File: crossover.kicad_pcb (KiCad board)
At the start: 2 copper layers, 99.7 x 90.8 mm, 86 parts, among them J1 Power In, J2 Line In, J3 Tweeter Out, J4 Sub Out, U1 TL072, U2 TL072, U3 TL072, U4 TL072, U5 TL072, U6 TL072, U7 TL072

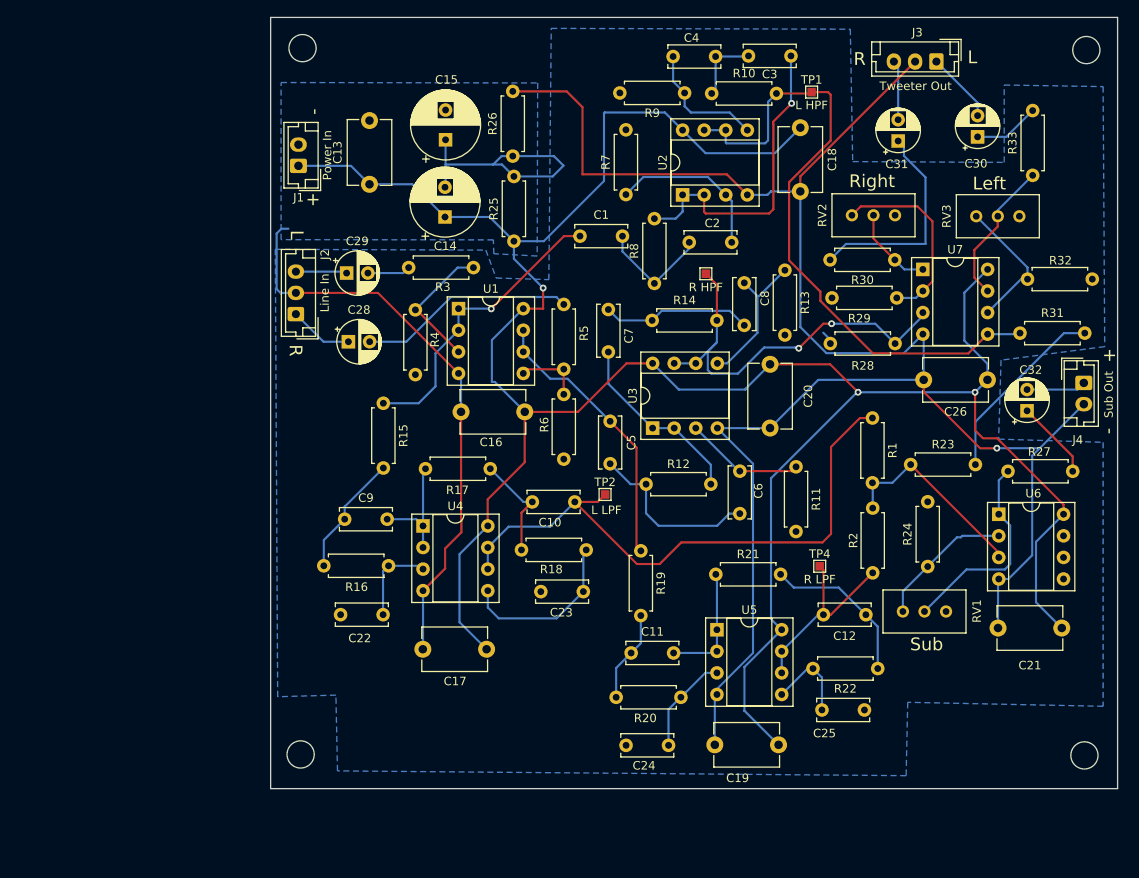
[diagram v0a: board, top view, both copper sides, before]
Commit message: Finish placing
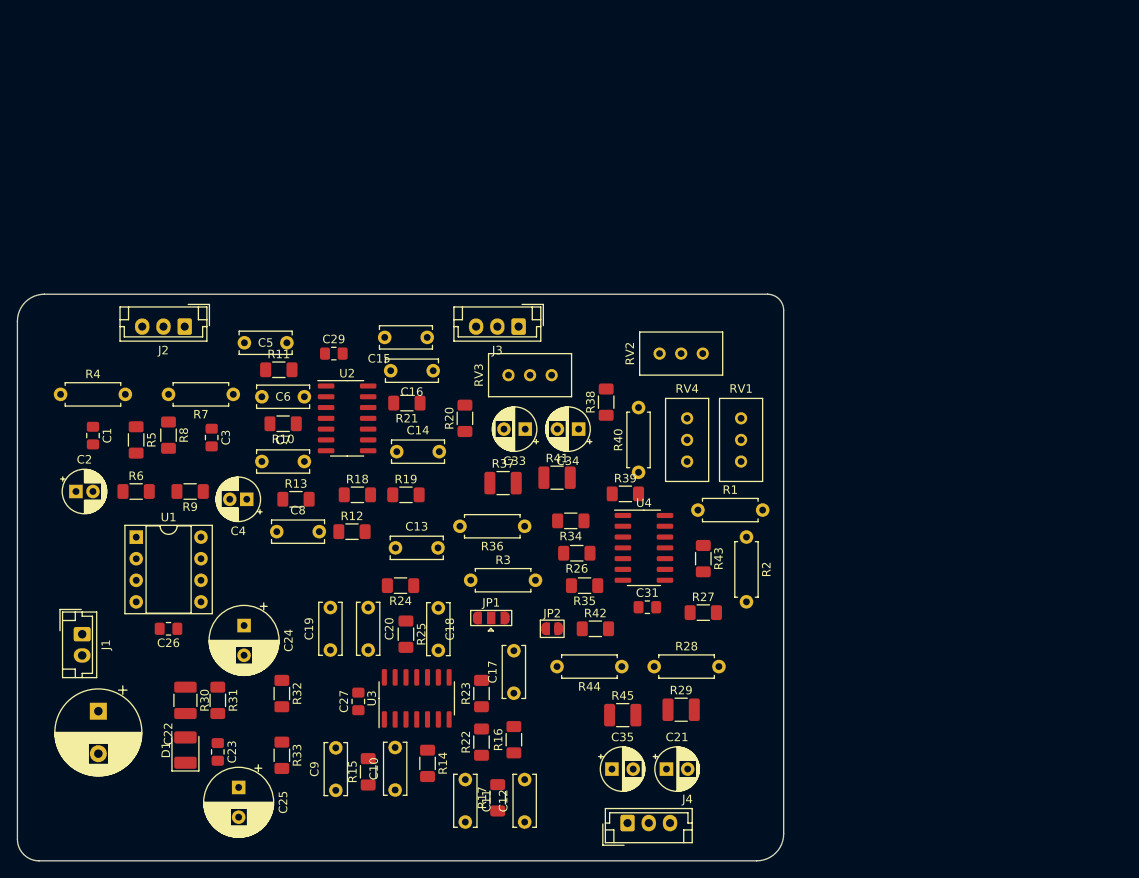
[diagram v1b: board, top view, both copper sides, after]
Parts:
- removed C28, C30, C32: 2.2u, Capacitor_THT:CP_Radial_D5.0mm_P2.50mm
- removed REF** (x4): MountingHole_3.2mm_M3, MountingHole:MountingHole_3.2mm_M3
- removed TP1: L HPF, TestPoint:TestPoint_Pad_1.0x1.0mm
- removed TP2: L LPF, TestPoint:TestPoint_Pad_1.0x1.0mm
- removed TP3: R HPF, TestPoint:TestPoint_Pad_1.0x1.0mm
- removed TP4: R LPF, TestPoint:TestPoint_Pad_1.0x1.0mm
- removed U5, U6, U7: TL072, Package_DIP:DIP-8_W7.62mm_Socket
- added C27: 100n, Capacitor_SMD:C_0805_2012Metric_Pad1.18x1.45mm_HandSolder, F.Cu at (73.1, 107.0)
- added C33: 2.2U, Capacitor_THT:CP_Radial_D5.0mm_P2.50mm, F.Cu at (92.8, 74.9)
- added C34: 2.2U, Capacitor_THT:CP_Radial_D5.0mm_P2.50mm, F.Cu at (99.1, 74.9)
- added C35: 2.2U, Capacitor_THT:CP_Radial_D5.0mm_P2.50mm, F.Cu at (103.0, 114.9)
- added D1: LED, LED_SMD:LED_1210_3225Metric_Pad1.42x2.65mm_HandSolder, F.Cu at (52.8, 112.7)
- added JP1: Sub Stereo/Mono, Jumper:SolderJumper-3_P1.3mm_Open_RoundedPad1.0x1.5mm, F.Cu at (88.8, 97.2)
- added JP2: Sub Mono, Jumper:SolderJumper-2_P1.3mm_Open_RoundedPad1.0x1.5mm, F.Cu at (96.0, 98.4)
- added R34: 10k, Resistor_SMD:R_1206_3216Metric_Pad1.30x1.75mm_HandSolder, F.Cu at (98.1, 85.7)
- added R35: 10K, Resistor_SMD:R_1206_3216Metric_Pad1.30x1.75mm_HandSolder, F.Cu at (99.8, 93.3)
- added R36: 100, Resistor_THT:R_Axial_DIN0207_L6.3mm_D2.5mm_P7.62mm_Horizontal, F.Cu at (92.7, 86.4)
- added R37: 4.7K, Resistor_SMD:R_1210_3225Metric_Pad1.30x2.65mm_HandSolder, F.Cu at (90.2, 81.3)
- added R38: 10k, Resistor_SMD:R_1206_3216Metric_Pad1.30x1.75mm_HandSolder, F.Cu at (102.3, 71.8)
- added R39: 10K, Resistor_SMD:R_1206_3216Metric_Pad1.30x1.75mm_HandSolder, F.Cu at (104.6, 82.5)
- added R40: 100, Resistor_THT:R_Axial_DIN0207_L6.3mm_D2.5mm_P7.62mm_Horizontal, F.Cu at (106.1, 80.0)
- added R41: 4.7K, Resistor_SMD:R_1210_3225Metric_Pad1.30x2.65mm_HandSolder, F.Cu at (96.5, 80.6)
- added R42: 10k, Resistor_SMD:R_1206_3216Metric_Pad1.30x1.75mm_HandSolder, F.Cu at (101.0, 98.4)
- added R43: 10K, Resistor_SMD:R_1206_3216Metric_Pad1.30x1.75mm_HandSolder, F.Cu at (113.7, 90.2)
- added R44: 100, Resistor_THT:R_Axial_DIN0207_L6.3mm_D2.5mm_P7.62mm_Horizontal, F.Cu at (104.1, 102.9)
- added R45: 4.7K, Resistor_SMD:R_1210_3225Metric_Pad1.30x2.65mm_HandSolder, F.Cu at (104.2, 108.6)
- added RV4: 10K, Potentiometer_THT:Potentiometer_Bourns_3386C_Horizontal, F.Cu at (111.8, 73.7)
- C1, C3: value 33nf -> 1n; footprint Capacitor_THT:C_Disc_D6.0mm_W2.5mm_P5.00mm -> Capacitor_SMD:C_0805_2012Metric_Pad1.18x1.45mm_HandSolder
- C10, C11, C12, C9: value 66nf -> 33nf
- C13, C17, C19: value 100n -> 33nf; footprint Capacitor_THT:C_Disc_D7.5mm_W5.0mm_P7.50mm -> Capacitor_THT:C_Disc_D6.0mm_W2.5mm_P5.00mm
- C14: value 10u -> 66nf; footprint Capacitor_THT:CP_Radial_D8.0mm_P3.50mm -> Capacitor_THT:C_Disc_D6.0mm_W2.5mm_P5.00mm
- C15: value 10u -> 33nf; footprint Capacitor_THT:CP_Radial_D8.0mm_P3.50mm -> Capacitor_THT:C_Disc_D6.0mm_W2.5mm_P5.00mm
- C16, C18, C20: value 100n -> 66nf; footprint Capacitor_THT:C_Disc_D7.5mm_W5.0mm_P7.50mm -> Capacitor_THT:C_Disc_D6.0mm_W2.5mm_P5.00mm
- C2, C4: value 33nf -> 4.7uF; footprint Capacitor_THT:C_Disc_D6.0mm_W2.5mm_P5.00mm -> Capacitor_THT:CP_Radial_D5.0mm_P2.00mm
- C21: value 100n -> 2.2U; footprint Capacitor_THT:C_Disc_D7.5mm_W5.0mm_P7.50mm -> Capacitor_THT:CP_Radial_D5.0mm_P2.50mm
- C22: value 33nf -> 1000uF; footprint Capacitor_THT:C_Disc_D6.0mm_W2.5mm_P5.00mm -> Capacitor_THT:CP_Radial_D10.0mm_P5.00mm
- C23: value 33nf -> 100n; footprint Capacitor_THT:C_Disc_D6.0mm_W2.5mm_P5.00mm -> Capacitor_SMD:C_0805_2012Metric_Pad1.18x1.45mm_HandSolder
- C24, C25: value 33nf -> 10u; footprint Capacitor_THT:C_Disc_D6.0mm_W2.5mm_P5.00mm -> Capacitor_THT:CP_Radial_D8.0mm_P3.50mm
- C26: footprint Capacitor_THT:C_Disc_D7.5mm_W5.0mm_P7.50mm -> Capacitor_SMD:C_0805_2012Metric_Pad1.18x1.45mm_HandSolder
- C29, C31: value 2.2u -> 100n; footprint Capacitor_THT:CP_Radial_D5.0mm_P2.50mm -> Capacitor_SMD:C_0805_2012Metric_Pad1.18x1.45mm_HandSolder
- J4: footprint Connector_JST:JST_EH_B2B-EH-A_1x02_P2.50mm_Vertical -> Connector_JST:JST_EH_B3B-EH-A_1x03_P2.50mm_Vertical
- R10, R12, R14, R16: value 27K -> 39K; footprint Resistor_THT:R_Axial_DIN0207_L6.3mm_D2.5mm_P7.62mm_Horizontal -> Resistor_SMD:R_1206_3216Metric_Pad1.30x1.75mm_HandSolder
- R11, R13: value 56K -> 20K; footprint Resistor_THT:R_Axial_DIN0207_L6.3mm_D2.5mm_P7.62mm_Horizontal -> Resistor_SMD:R_1206_3216Metric_Pad1.30x1.75mm_HandSolder
- R15, R17, R18, R19, R20, R21, R22: value 27K -> 20K; footprint Resistor_THT:R_Axial_DIN0207_L6.3mm_D2.5mm_P7.62mm_Horizontal -> Resistor_SMD:R_1206_3216Metric_Pad1.30x1.75mm_HandSolder
- R23: value 10k -> 20K; footprint Resistor_THT:R_Axial_DIN0207_L6.3mm_D2.5mm_P7.62mm_Horizontal -> Resistor_SMD:R_1206_3216Metric_Pad1.30x1.75mm_HandSolder
- R24: value 5k -> 20K; footprint Resistor_THT:R_Axial_DIN0207_L6.3mm_D2.5mm_P7.62mm_Horizontal -> Resistor_SMD:R_1206_3216Metric_Pad1.30x1.75mm_HandSolder
- R25: value 10K -> 20K; footprint Resistor_THT:R_Axial_DIN0207_L6.3mm_D2.5mm_P7.62mm_Horizontal -> Resistor_SMD:R_1206_3216Metric_Pad1.30x1.75mm_HandSolder
- R26: value 10K -> 10k; footprint Resistor_THT:R_Axial_DIN0207_L6.3mm_D2.5mm_P7.62mm_Horizontal -> Resistor_SMD:R_1206_3216Metric_Pad1.30x1.75mm_HandSolder
- R27, R33: value 100 -> 10K; footprint Resistor_THT:R_Axial_DIN0207_L6.3mm_D2.5mm_P7.62mm_Horizontal -> Resistor_SMD:R_1206_3216Metric_Pad1.30x1.75mm_HandSolder
- R28: value 10k -> 100
- R29: value 5k -> 4.7K; footprint Resistor_THT:R_Axial_DIN0207_L6.3mm_D2.5mm_P7.62mm_Horizontal -> Resistor_SMD:R_1210_3225Metric_Pad1.30x2.65mm_HandSolder
- R3: value 1K -> 100
- R30: value 100 -> 2.2K; footprint Resistor_THT:R_Axial_DIN0207_L6.3mm_D2.5mm_P7.62mm_Horizontal -> Resistor_SMD:R_1210_3225Metric_Pad1.30x2.65mm_HandSolder
- R31: value 10k -> 1K; footprint Resistor_THT:R_Axial_DIN0207_L6.3mm_D2.5mm_P7.62mm_Horizontal -> Resistor_SMD:R_1206_3216Metric_Pad1.30x1.75mm_HandSolder
- R32: value 5k -> 10K; footprint Resistor_THT:R_Axial_DIN0207_L6.3mm_D2.5mm_P7.62mm_Horizontal -> Resistor_SMD:R_1206_3216Metric_Pad1.30x1.75mm_HandSolder
- R4: value 100K -> 100
- R5: value 1K -> 22K; footprint Resistor_THT:R_Axial_DIN0207_L6.3mm_D2.5mm_P7.62mm_Horizontal -> Resistor_SMD:R_1206_3216Metric_Pad1.30x1.75mm_HandSolder
- R6: value 100K -> 22K; footprint Resistor_THT:R_Axial_DIN0207_L6.3mm_D2.5mm_P7.62mm_Horizontal -> Resistor_SMD:R_1206_3216Metric_Pad1.30x1.75mm_HandSolder
- R7: value 56K -> 100
- R8: value 27K -> 22K; footprint Resistor_THT:R_Axial_DIN0207_L6.3mm_D2.5mm_P7.62mm_Horizontal -> Resistor_SMD:R_1206_3216Metric_Pad1.30x1.75mm_HandSolder
- R9: value 56K -> 22K; footprint Resistor_THT:R_Axial_DIN0207_L6.3mm_D2.5mm_P7.62mm_Horizontal -> Resistor_SMD:R_1206_3216Metric_Pad1.30x1.75mm_HandSolder
- U2, U3, U4: value TL072 -> TL074; footprint Package_DIP:DIP-8_W7.62mm_Socket -> Package_SO:SOIC-14_3.9x8.7mm_P1.27mm
- moved R33 111.6 mm to (64.1, 113.3), turned to -90 degrees
- moved R31 103.8 mm to (56.6, 106.8), turned to -90 degrees
- moved C26 100.7 mm to (50.8, 98.4)
- moved R32 100.4 mm to (64.1, 106.0), turned to -90 degrees
- moved R30 98.3 mm to (52.8, 106.8), turned to -90 degrees
- moved C3 81.6 mm to (55.9, 75.9), turned to -90 degrees
- moved C2 77.9 mm to (39.9, 82.3)
- moved C4 75.9 mm to (60.0, 83.2)
- moved C18 74.8 mm to (82.5, 101.0), turned to 90 degrees
- moved R9 74.7 mm to (53.3, 82.3)
- moved J4 74.6 mm to (104.8, 121.3), turned to 0 degrees
- moved C25 74.2 mm to (59.1, 117.1), turned to -90 degrees
- moved R10 63.7 mm to (64.3, 74.3), turned to 180 degrees
- moved R13 63.5 mm to (65.8, 83.2), turned to 0 degrees
- moved C31 62.3 mm to (107.1, 95.9), turned to 0 degrees
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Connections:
- C1 pad 1: /Left HPF/in -> Net-(C1-Pad1)
- C1 pad 2: Net-(C1-Pad2) -> VDD
- C10 pad 2: /Left LPF/out -> Net-(U3A-+)
- C11 pad 1: Net-(C11-Pad1) -> /Right HPF/HPF Stage 2/in
- C11 pad 2: /Right LPF/LPF Stage 1/out -> Net-(C11-Pad2)
- C12 pad 1: Net-(C12-Pad1) -> Net-(C11-Pad2)
- C12 pad 2: /Right LPF/out -> Net-(U3B-+)
- C13 pad 1: VCC -> GNDREF
- C13 pad 2: VDD -> Net-(U2C-+)
- C14 pad 1: VCC -> Net-(C14-Pad1)
- C14 pad 2: GNDREF -> /Left LPF/LPF Stage 1/out
- C15 pad 2: VDD -> Net-(U2D-+)
- C16 pad 1: VCC -> Net-(C16-Pad1)
- C16 pad 2: VDD -> /Left LPF/out
- C17 pad 1: VCC -> GNDREF
- C17 pad 2: VDD -> Net-(U3C-+)
- C18 pad 1: VCC -> Net-(C18-Pad1)
- C18 pad 2: VDD -> /Right LPF/LPF Stage 1/out
- C19 pad 1: VCC -> GNDREF
- C19 pad 2: VDD -> Net-(U3D-+)
- C2 pad 1: Net-(C1-Pad2) -> Net-(C1-Pad1)
- C2 pad 2: Net-(C2-Pad2) -> Net-(U1A-+)
- C20 pad 1: VCC -> Net-(C20-Pad1)
- C20 pad 2: VDD -> /Right LPF/out
- C21 pad 1: VCC -> Net-(C21-Pad1)
- C21 pad 2: VDD -> /sub gain/out
- C22 pad 1: GNDREF -> VCC
- C22 pad 2: Net-(C22-Pad2) -> VDD
- C23 pad 1: GNDREF -> Net-(C23-Pad1)
- C23 pad 2: Net-(C23-Pad2) -> VDD
- C24 pad 1: GNDREF -> VCC
- C24 pad 2: Net-(C24-Pad2) -> GNDREF
- C25 pad 2: Net-(C25-Pad2) -> VDD
- C29 pad 1: Net-(C29-Pad1) -> VCC
- C29 pad 2: /Left Input Buffer/In -> VDD
- C3 pad 1: /Left HPF/HPF Stage 2/in -> Net-(C3-Pad1)
- C3 pad 2: Net-(C3-Pad2) -> VDD
- C31 pad 1: /Right gain/out -> VCC
- C31 pad 2: Net-(C31-Pad2) -> VDD
- C4 pad 1: Net-(C3-Pad2) -> Net-(C3-Pad1)
- C4 pad 2: Net-(C4-Pad2) -> Net-(U1B-+)
- C5 pad 1: /Right HPF/in -> /Left HPF/in
- C6 pad 2: Net-(C6-Pad2) -> Net-(U2A-+)
- C7 pad 1: /Right HPF/HPF Stage 2/in -> /Left HPF/HPF Stage 2/in
- C8 pad 2: Net-(C8-Pad2) -> Net-(U2B-+)
- C9 pad 1: Net-(C9-Pad1) -> /Right HPF/in
- C9 pad 2: /Left LPF/LPF Stage 1/out -> Net-(C10-Pad1)
- J2 pad 1: Net-(C28-Pad1) -> /Right Input Buffer/In
- J2 pad 3: Net-(C29-Pad1) -> /Left Input Buffer/In
- J3 pad 1: Net-(C30-Pad2) -> /Left Gain/out
- J3 pad 3: Net-(C31-Pad2) -> /Right gain/out
- J4 pad 1: Net-(C32-Pad2) -> /Sub Gain Stereo/out
- R10 pad 1: Net-(C3-Pad2) -> Net-(U2A-+)
- R10 pad 2: /Left Gain/in -> GNDREF
- R11 pad 1: Net-(C6-Pad2) -> Net-(C5-Pad2)
- R11 pad 2: GNDREF -> /Left HPF/HPF Stage 2/in
- R12 pad 1: Net-(C5-Pad2) -> Net-(U2B-+)
- R12 pad 2: /Right HPF/HPF Stage 2/in -> GNDREF
- R13 pad 1: Net-(C8-Pad2) -> Net-(C7-Pad2)
- R13 pad 2: GNDREF -> /Left Gain/in
- R14 pad 1: Net-(C7-Pad2) -> Net-(U3A-+)
- R14 pad 2: /Right HPF/out -> GNDREF
- R15 pad 1: /Left HPF/in -> Net-(C10-Pad1)
- R15 pad 2: Net-(C9-Pad1) -> /Right HPF/HPF Stage 2/in
- R16 pad 1: Net-(C9-Pad1) -> Net-(U3B-+)
- R16 pad 2: Net-(C22-Pad2) -> GNDREF
- R17 pad 1: /Left LPF/LPF Stage 1/out -> Net-(C11-Pad2)
- R17 pad 2: Net-(C10-Pad1) -> /Right HPF/out
- R18 pad 1: Net-(C10-Pad1) -> /Left HPF/in
- R18 pad 2: Net-(C23-Pad2) -> Net-(C14-Pad1)
- R19 pad 1: /Right HPF/in -> Net-(C14-Pad1)
- R19 pad 2: Net-(C11-Pad1) -> Net-(U2C-+)
- R2 pad 2: /Right LPF/out -> Net-(JP1-A)
- R20 pad 1: Net-(C11-Pad1) -> /Left LPF/LPF Stage 1/out
- R20 pad 2: Net-(C24-Pad2) -> Net-(C16-Pad1)
- R21 pad 1: /Right LPF/LPF Stage 1/out -> Net-(C16-Pad1)
- R21 pad 2: Net-(C12-Pad1) -> Net-(U2D-+)
- R22 pad 1: Net-(C12-Pad1) -> /Right HPF/in
- R22 pad 2: Net-(C25-Pad2) -> Net-(C18-Pad1)
- R23 pad 1: /sub gain/in -> Net-(C18-Pad1)
- R23 pad 2: GNDREF -> Net-(U3C-+)
- R24 pad 1: Net-(R24-Pad1) -> /Right LPF/LPF Stage 1/out
- R24 pad 2: GNDREF -> Net-(C20-Pad1)
- R25 pad 1: VCC -> Net-(C20-Pad1)
- R25 pad 2: GNDREF -> Net-(U3D-+)
- R26 pad 1: GNDREF -> /sub gain/in
- R26 pad 2: VDD -> GNDREF
- R27 pad 1: Net-(R27-Pad1) -> Net-(U4C--)
- R27 pad 2: /sub gain/out -> GNDREF
- R28 pad 1: /Right HPF/out -> Net-(R28-Pad1)
- R28 pad 2: GNDREF -> Net-(C21-Pad1)
- R29 pad 1: Net-(R29-Pad1) -> /sub gain/out
- R29 pad 2: GNDREF -> VDD
- R3 pad 1: Net-(R3-Pad1) -> Net-(JP1-B)
- R3 pad 2: /Left Input Buffer/In -> /Sub Gain Stereo/in
- R30 pad 1: Net-(R30-Pad1) -> VCC
- R30 pad 2: /Right gain/out -> Net-(D1-A)
- R31 pad 1: /Left Gain/in -> VCC
- R31 pad 2: GNDREF -> Net-(C23-Pad1)
- R32 pad 1: Net-(R32-Pad1) -> VCC
- R33 pad 1: Net-(R33-Pad1) -> GNDREF
- R33 pad 2: /Left Gain/out -> VDD
- R4 pad 1: Net-(R3-Pad1) -> /Left Input Buffer/In
- R4 pad 2: GNDREF -> Net-(C1-Pad1)
- R5 pad 1: Net-(R5-Pad1) -> Net-(C1-Pad1)
- R5 pad 2: /Right Input Buffer/In -> VDD
- R6 pad 1: Net-(R5-Pad1) -> Net-(U1A-+)
- R7 pad 1: Net-(C2-Pad2) -> /Right Input Buffer/In
- R7 pad 2: GNDREF -> Net-(C3-Pad1)
- R8 pad 1: Net-(C1-Pad2) -> Net-(C3-Pad1)
- R8 pad 2: /Left HPF/HPF Stage 2/in -> VDD
- R9 pad 1: Net-(C4-Pad2) -> Net-(U1B-+)
- RV1 pad 1: Net-(R24-Pad1) -> Net-(U4C--)
- RV1 pad 2: Net-(R27-Pad1) -> Net-(R28-Pad1)
- RV2 pad 1: Net-(R29-Pad1) -> Net-(U4B--)
- RV2 pad 2: Net-(R30-Pad1) -> Net-(R36-Pad1)
- RV3 pad 1: Net-(R32-Pad1) -> Net-(U4A--)
- RV3 pad 2: Net-(R33-Pad1) -> Net-(R40-Pad1)
- U1 pad 3: Net-(R3-Pad1) -> Net-(U1A-+)
- U1 pad 5: Net-(R5-Pad1) -> Net-(U1B-+)
- U2 pad 3: Net-(C2-Pad2) -> Net-(U2A-+)
- U2 pad 4: VDD -> VCC
- U2 pad 5: Net-(C4-Pad2) -> Net-(U2B-+)
- U2 pad 8: VCC -> /Left LPF/LPF Stage 1/out
- U3 pad 3: Net-(C6-Pad2) -> Net-(U3A-+)
- U3 pad 4: VDD -> VCC
- U3 pad 5: Net-(C8-Pad2) -> Net-(U3B-+)
- U3 pad 8: VCC -> /Right LPF/LPF Stage 1/out
- U4 pad 1: /Left LPF/LPF Stage 1/out -> Net-(R40-Pad1)
- U4 pad 2: /Left LPF/LPF Stage 1/out -> Net-(U4A--)
- U4 pad 3: Net-(C22-Pad2) -> /Left Gain/in
- U4 pad 4: VDD -> VCC
- U4 pad 5: Net-(C23-Pad2) -> /Right HPF/out
- U4 pad 6: /Left LPF/out -> Net-(U4B--)
- U4 pad 7: /Left LPF/out -> Net-(R36-Pad1)
- U4 pad 8: VCC -> Net-(R28-Pad1)
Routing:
- net VCC: track 298.6 -> 0.00 mm, vias 3 -> 0
- net VDD: track 287.3 -> 0.00 mm, vias 1 -> 0
- net /Left Gain/in: track 76.5 -> 0.00 mm
- net /Left LPF/out: track 70.1 -> 0.00 mm
- net GNDREF: track 53.6 -> 0.00 mm
- net /Right HPF/out: track 49.1 -> 0.00 mm, vias 2 -> 0
- net /Left HPF/HPF Stage 2/in: track 37.6 -> 0.00 mm, vias 1 -> 0
- net /Left HPF/in: track 35.1 -> 0.00 mm, vias 1 -> 0
- net /Right HPF/in: track 32.9 -> 0.00 mm
- net /Right gain/out: track 25.5 -> 0.00 mm
- net /Right Input Buffer/In: track 25.4 -> 0.00 mm
- net Net-(R27-Pad1): track 24.3 -> 0.00 mm
- net /sub gain/in: track 23.6 -> 0.00 mm
- net /Right LPF/out: track 23.0 -> 0.00 mm
- net Net-(R29-Pad1): track 22.7 -> 0.00 mm
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- removed copper zone on B.Cu, net GNDREF
- removed copper zone on B.Cu, net VDD
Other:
- board size 99.7 x 90.8 mm -> 90.2 x 66.7 mm
- rule pad_to_mask_clearance: 0 -> 0.05
- board text removed: "+"
- board text removed: "-"
- board text removed: "Audio Crossover v1.0 Circuit: https://sound-au.com/project09.htm"
- board text removed: "L"
- board text removed: "Left"
- board text removed: "R"
- board text removed: "Right"
- board text removed: "Sub"
